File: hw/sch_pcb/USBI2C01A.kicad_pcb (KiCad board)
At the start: 2 copper layers, 30 x 40.1 mm, 26 parts, among them P1 750mA, X1 CP2112, X2 USB_B, X3 SROUB3M, X4 SROUB3M, X5 SROUB3M, X6 SROUB3M

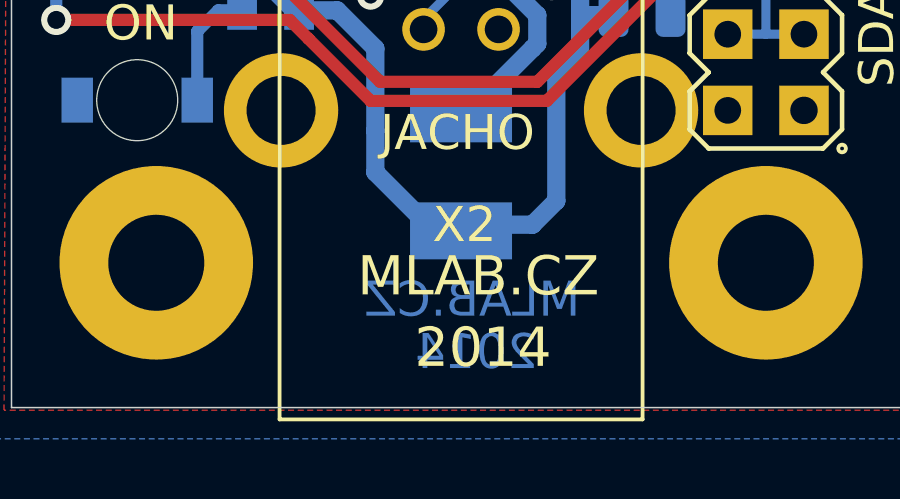
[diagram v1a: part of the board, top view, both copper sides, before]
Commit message: Uprava projektovych dat
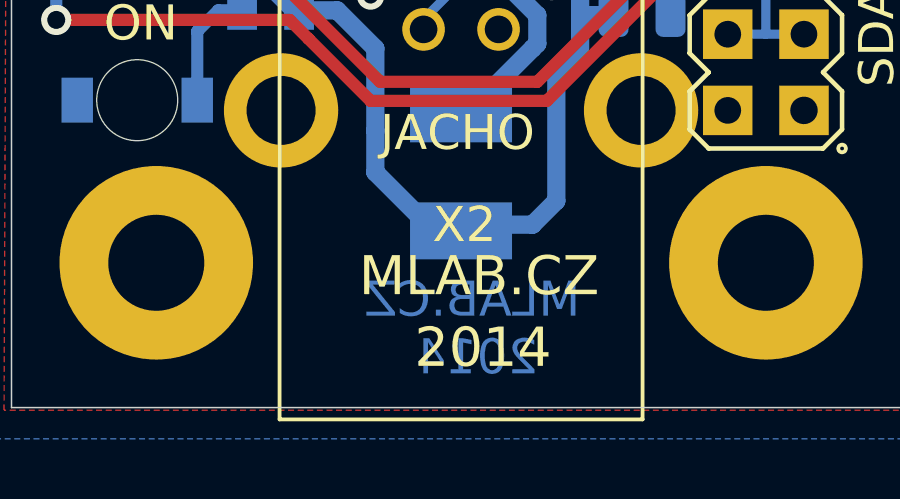
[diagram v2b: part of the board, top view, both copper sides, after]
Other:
- rule pad_to_mask_clearance: 0 -> 0.2
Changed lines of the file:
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@@
   )
   (paper "A4")
+  (title_block
+    (rev "I2CUSB01A")
+    (company "MLAB")
+  )
   (layers
     (0 "F.Cu" signal)
@@
     (48 "B.Fab" user)
     (49 "F.Fab" user)
-    (50 "User.1" user)
-    (51 "User.2" user)
-    (52 "User.3" user)
-    (53 "User.4" user)
-    (54 "User.5" user)
-    (55 "User.6" user)
-    (56 "User.7" user)
-    (57 "User.8" user)
-    (58 "User.9" user)
   )
   (setup
-    (pad_to_mask_clearance 0)
+    (stackup
+      (layer "F.SilkS" (type "Top Silk Screen") (color "Black"))
+      (layer "F.Paste" (type "Top Solder Paste"))
+      (layer "F.Mask" (type "Top Solder Mask") (color "White") (thickness 0.01))
+      (layer "F.Cu" (type "copper") (thickness 0.035))
+      (layer "dielectric 1" (type "core") (thickness 1.51) (material "FR4") (epsilon_r 4.5) (loss_tangent 0.02))
+      (layer "B.Cu" (type "copper") (thickness 0.035))
+      (layer "B.Mask" (type "Bottom Solder Mask") (color "White") (thickness 0.01))
+      (layer "B.Paste" (type "Bottom Solder Paste"))
+      (layer "B.SilkS" (type "Bottom Silk Screen") (color "Black"))
+      (copper_finish "HAL lead-free")
+      (dielectric_constraints no)
+      (castellated_pads yes)
+    )
+    (pad_to_mask_clearance 0.2)
+    (grid_origin 133.5151 125.0696)
     (pcbplotparams
       (layerselection 0x00010fc_ffffffff)
@@
     (effects (font (size 1.1684 1.1684) (thickness 0.1016)) (justify left bottom mirror))
   )
-  (gr_text "2014" (at 151.0411 123.89485) (layer "B.Cu")
+  (gr_text "2014" (at 151.0651 124.0696) (layer "B.Cu")
     (effects (font (size 1.1684 1.1684) (thickness 0.1016)) (justify left bottom mirror))
   )
@@
   )
   (gr_text "MLAB.CZ" (at 153.10485 119.9261) (layer "F.SilkS")
-    (effects (font (size 1.308608 1.308608) (thickness 0.113792)) (justify right top))
+    (effects (font (size 1.3 1.3) (thickness 0.2)) (justify right top))
   )
   (gr_text "7" (at 142.94485 94.2086) (layer "F.SilkS")
@@
   (gr_text "3.3V" (at 148.65985 105.16235) (layer "F.SilkS")
     (effects (font (size 1.1684 1.1684) (thickness 0.1016)) (justify left bottom))
+  )
+  (dimension (type aligned) (layer "Dwgs.User")
+    (pts (xy 163.4871 84.9376) (xy 133.5151 84.9376))
+    (height 4.468)
+    (gr_text "30,0 mm" (at 148.5011 78.6696) (layer "Dwgs.User")
+      (effects (font (size 1.5 1.5) (thickness 0.3)))
+    )
+    (format (units 3) (units_format 1) (precision 1))
+    (style (thickness 0.2) (arrow_length 1.27) (text_position_mode 0) (extension_height 0.58642) (extension_offset 0.5) keep_text_aligned)
+  )
+  (dimension (type aligned) (layer "Dwgs.User")
+    (pts (xy 163.4871 125.0696) (xy 163.4871 84.9376))
+    (height 7.178)
+    (gr_text "40,1 mm" (at 168.8651 105.0036 90) (layer "Dwgs.User")
+      (effects (font (size 1.5 1.5) (thickness 0.3)))
+    )
+    (format (units 3) (units_format 1) (precision 1))
+    (style (thickness 0.2) (arrow_length 1.27) (text_position_mode 0) (extension_height 0.58642) (extension_offset 0.5) keep_text_aligned)
   )
   (dimension (type aligned) (layer "Cmts.User")
@@
       (effects (font (size 1 1) (thickness 0.15)))
     )
-    (format (units 2) (units_format 1) (precision 1))
-    (style (thickness 0.1) (arrow_length 1.27) (text_position_mode 0) (extension_height 0.58642) (extension_offset 0) keep_text_aligned)
-  )
-  (dimension (type aligned) (layer "Cmts.User")
-    (pts (xy 163.4871 125.0696) (xy 163.4871 84.9376))
-    (height 5.969)
-    (gr_text "40.1 mm" (at 168.3061 105.0036 90) (layer "Cmts.User")
-      (effects (font (size 1 1) (thickness 0.15)))
-    )
